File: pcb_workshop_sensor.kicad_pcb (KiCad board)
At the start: 2 copper layers, 41.3 x 47 mm, 27 parts, among them IC1 ATTINY841-SSU, J1 USB, P1 BSL, P2 BSL, P3 ISP, U1 MSP430FR5738, X1 32768Hz, X2 12MHz

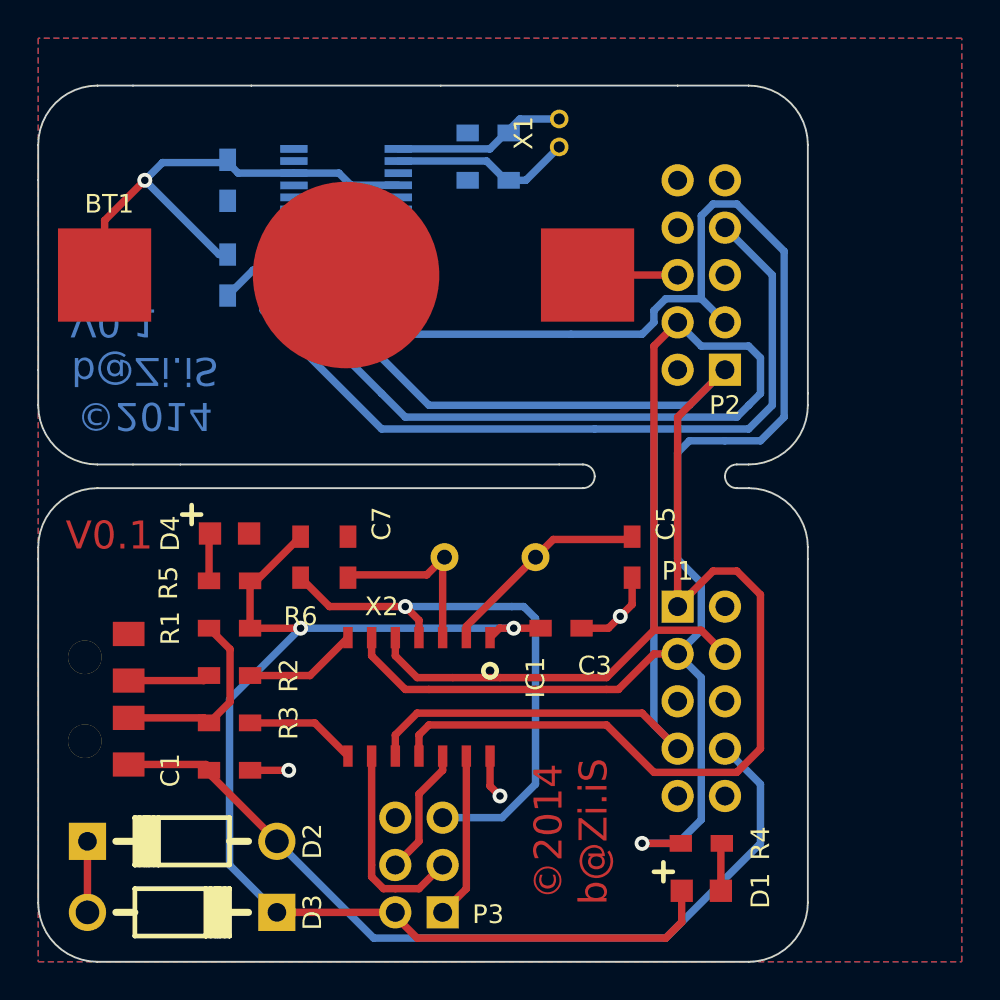
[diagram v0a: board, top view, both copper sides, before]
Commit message: v1.0
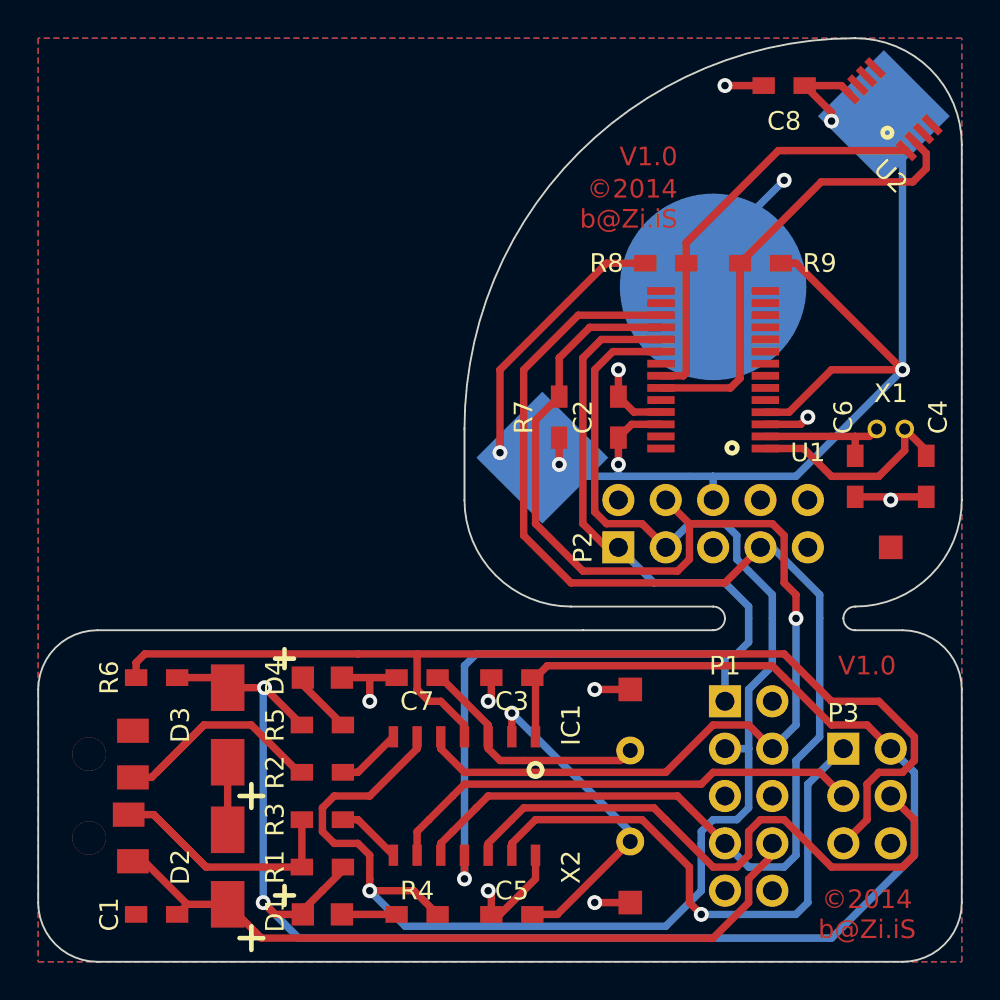
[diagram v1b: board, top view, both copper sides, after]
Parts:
- added C8: 0.1µF, workshop:0603, F.Cu at (60.3, 128.3)
- added R8: 10k, workshop:0603, F.Cu at (59.1, 137.8)
- added R9: 10k, workshop:0603, F.Cu at (54.0, 137.8)
- added U2: TMP275, workshop:MSOP-8, F.Cu at (66.0, 129.5)
- BT1: moved to B.Cu
- C2, C4, C6, R7, U1: moved to F.Cu
- D2, D3: footprint Diodes_ThroughHole:Diode_DO-41_SOD81_Horizontal_RM10 -> workshop:Diode-SMA_Standard
- moved C4 29.9 mm to (67.9, 149.2), turned to 90 degrees
- moved C6 25.3 mm to (64.1, 149.2), turned to 90 degrees
- moved C2 24.5 mm to (51.4, 146.1), turned to 90 degrees
- moved P3 24.3 mm to (64.8, 166.4), turned to 270 degrees
- moved X1 23.8 mm to (66.0, 146.7), turned to 180 degrees
- moved U1 21.1 mm to (56.5, 143.5), turned to 90 degrees
- moved D1 20.4 mm to (35.6, 172.7)
- moved C5 20.2 mm to (45.7, 172.7), turned to 0 degrees
- moved BT1 19.7 mm to (56.5, 139.1), turned to 45 degrees
- moved R7 19.3 mm to (48.3, 146.1), turned to 270 degrees
- moved R4 15.7 mm to (40.6, 172.7), turned to 180 degrees
- moved X2 14.9 mm to (52.1, 166.4), turned to 90 degrees
- moved R1 13.7 mm to (35.6, 170.2)
- moved P2 13.4 mm to (56.5, 151.8), turned to 0 degrees
- moved D3 10.3 mm to (30.5, 162.6), turned to 90 degrees
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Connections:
- U1 pad 22: (no net) -> /SDA
- U1 pad 23: (no net) -> /SCL
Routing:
- net +BATT: track 33.6 -> 89.3 mm, vias 1 -> 5
- net VCC: track 65.8 -> 95.0 mm
- net /AVR_RST: track 30.1 -> 59.1 mm, vias 1 -> 0
- net /MOSI: track 6.89 -> 32.4 mm
- net GND: track 9.88 -> 34.9 mm, vias 3 -> 10
- net /SCL: track 0.00 -> 24.4 mm
- net /SDA: track 0.00 -> 22.3 mm
- net /AVR_RX: track 78.2 -> 57.1 mm, vias 0 -> 1
- net /MISO: track 8.91 -> 29.6 mm, vias 0 -> 1
- net /AVR_TX: track 99.8 -> 81.2 mm
- net /SCK: track 11.1 -> 26.0 mm
- net /AVR_DTR: track 79.7 -> 66.9 mm, vias 0 -> 1
- net Net-(J1-Pad3): track 4.09 -> 15.1 mm
- net Net-(J1-Pad2): track 10.1 -> 17.0 mm
- net /AVR_RTS: track 79.8 -> 73.3 mm
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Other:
- board size 41.3 x 47 mm -> 49.5 x 49.5 mm
- board text added: "V1.0"
- board text removed: "V0.1"
